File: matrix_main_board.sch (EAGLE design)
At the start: 137 parts, among them IC1 MKE02_44PIN, IC2 24AA01SM, IC3 74HC595D, IC4 74HC595D, IC5 74HC595D, IC6 74HC595D, IC7 NPIC6C596, IC8 NPIC6C596, IC9 W25Q128, U1 RP2040

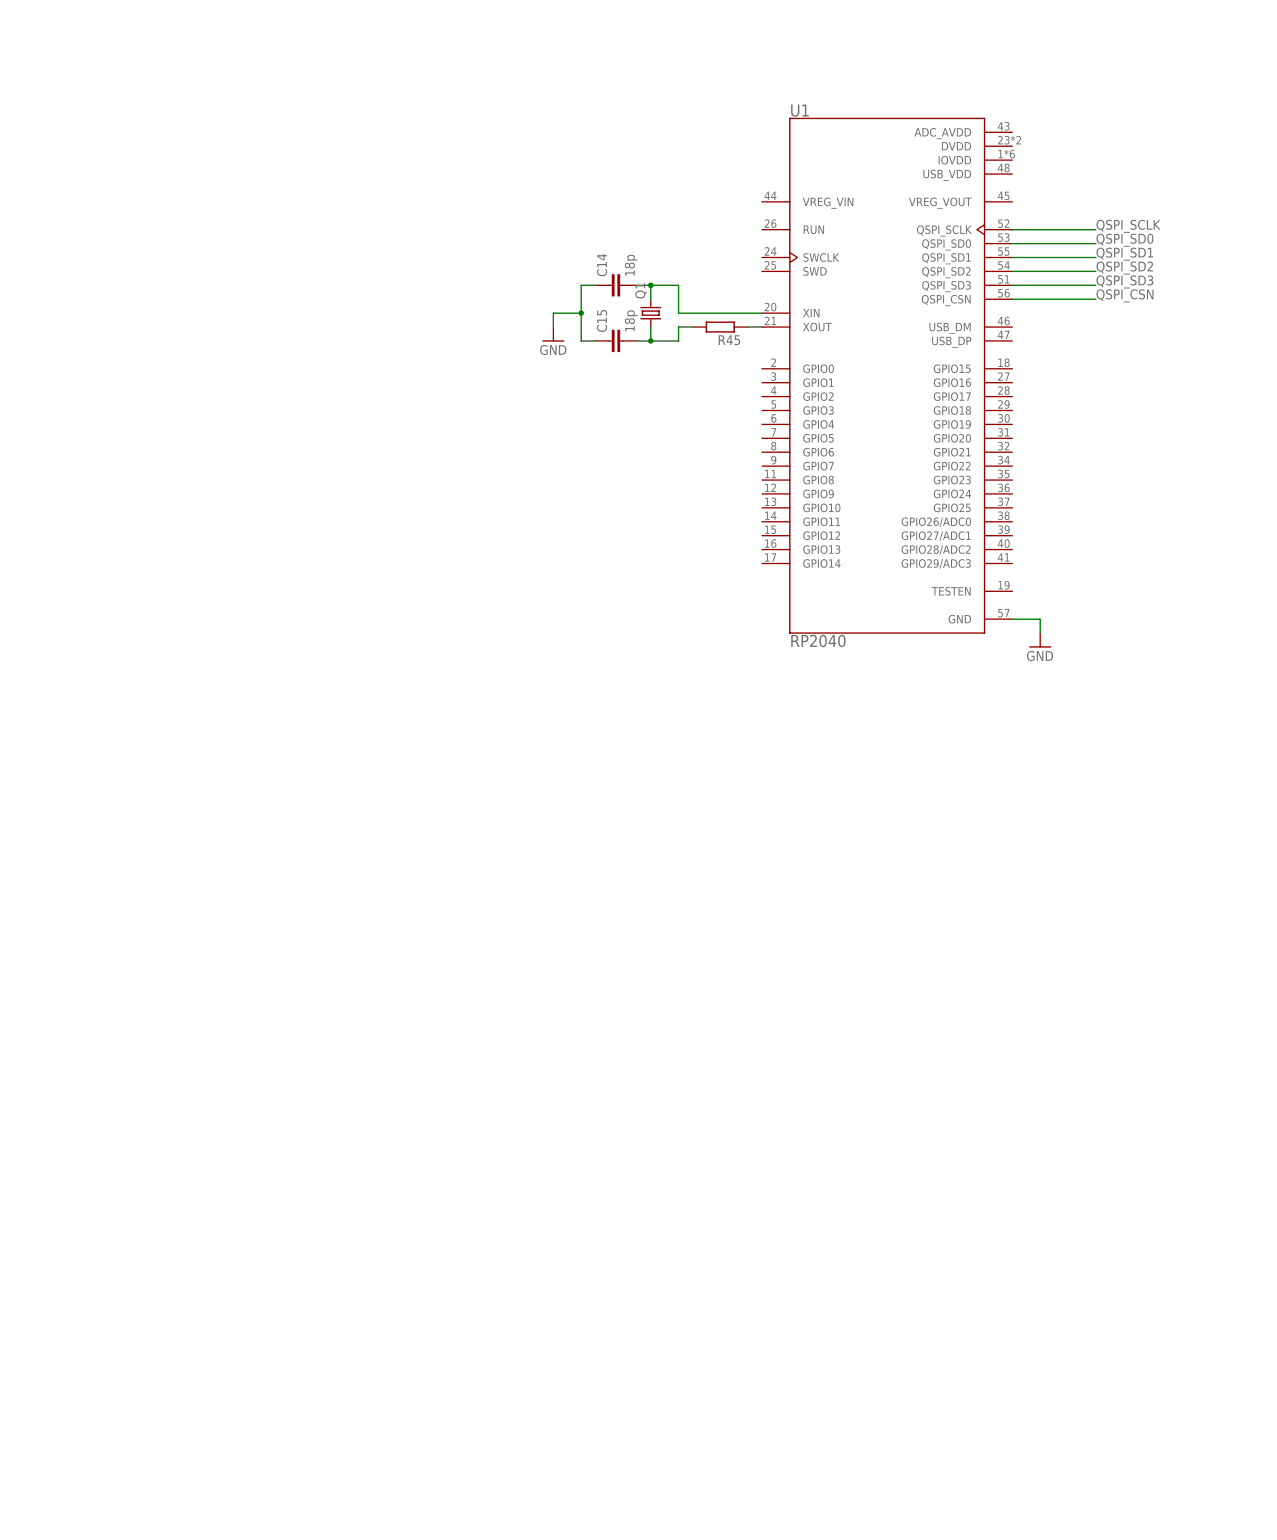
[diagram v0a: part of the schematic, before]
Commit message: ASAS
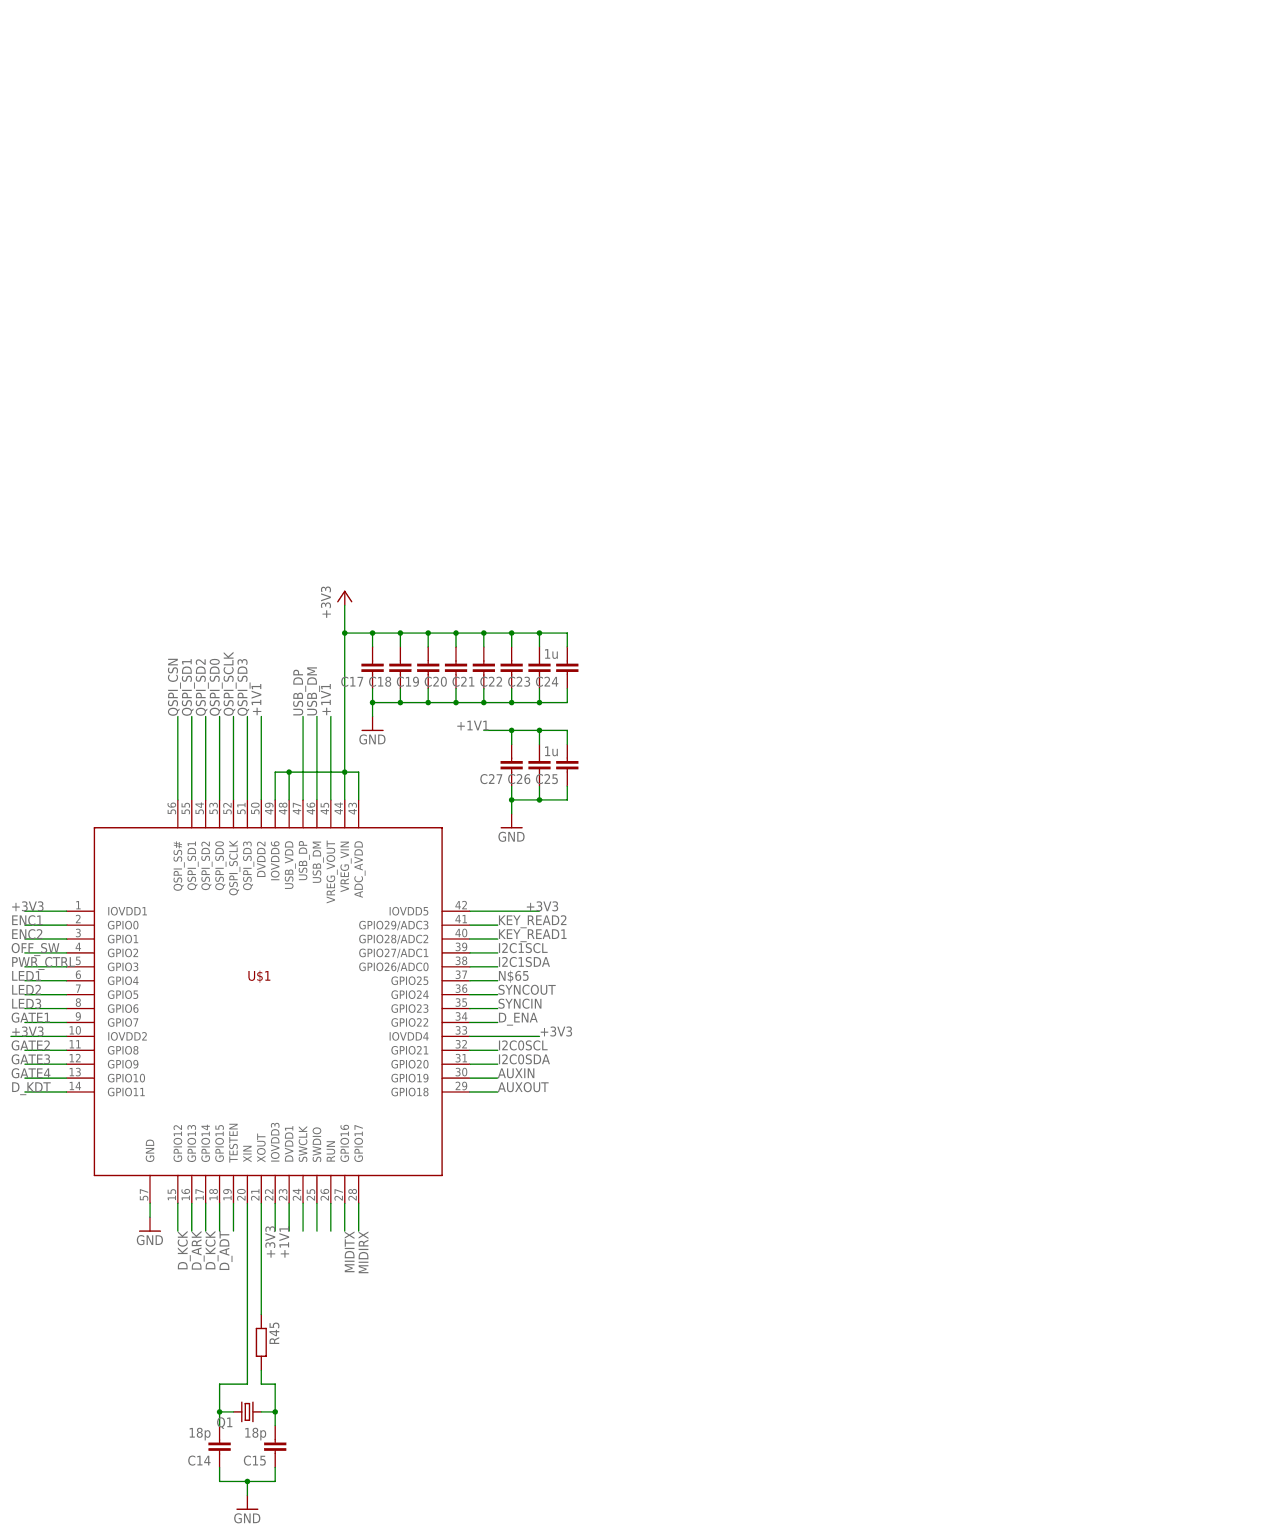
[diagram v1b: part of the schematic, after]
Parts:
- removed U1: RP2040, RP2040:RP2040
- added C17, C18, C19, C20, C21, C22, C23, C26, C27: (no value), rcl:C-EUC0805
- added C24, C25: 1u, rcl:C-EUC0805
- added U$1: RP2040, jason_eagle6:RP2040
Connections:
- new net +1V1: C25.2, C26.2, C27.2, U$1.DVDD1, U$1.DVDD2, U$1.VREG_VOUT
- new net +3V3: C17.2, C18.2, C19.2, C20.2, C21.2, C22.2, C23.2, C24.2, U$1.ADC_AVDD, U$1.IOVDD1, U$1.IOVDD2, U$1.IOVDD3, U$1.IOVDD4, U$1.IOVDD5, U$1.IOVDD6, U$1.USB_VDD, U$1.VREG_VIN
- new net N$44: U$1.TESTEN
- new net N$45: U$1.SWCLK
- new net N$46: U$1.SWDIO
- new net N$47: U$1.RUN
- new net N$65: U$1.GPIO25
- new net USB_DM: U$1.USB_DM
- new net USB_DP: U$1.USB_DP
- net AUXIN: now also U$1.GPIO19
- net AUXOUT: now also U$1.GPIO18
- net D_ADT: now also U$1.GPIO15
- net D_ARK: now also U$1.GPIO13
- net D_ENA: now also U$1.GPIO22
- net D_KCK: now also U$1.GPIO12, U$1.GPIO14
- net D_KDT: now also U$1.GPIO11
- net ENC1: now also U$1.GPIO0
- net ENC2: now also U$1.GPIO1
- net GATE1: now also U$1.GPIO7
- net GATE2: now also U$1.GPIO8
- net GATE3: now also U$1.GPIO9
- net GATE4: now also U$1.GPIO10
- net GND: now also C17.1, C18.1, C19.1, C20.1, C21.1, C22.1, C23.1, C24.1, C25.1, C26.1, C27.1, U$1.GND; no longer U1.GND
- net I2C0SCL: now also U$1.GPIO21
- net I2C0SDA: now also U$1.GPIO20
- net I2C1SCL: now also U$1.GPIO27/ADC1
- net I2C1SDA: now also U$1.GPIO26/ADC0
- net KEY_READ1: now also U$1.GPIO28/ADC2
- net KEY_READ2: now also U$1.GPIO29/ADC3
- net LED1: now also U$1.GPIO4
- net LED2: now also U$1.GPIO5
- net LED3: now also U$1.GPIO6
- net MIDIRX: now also U$1.GPIO17
- net MIDITX: now also U$1.GPIO16
- net N$10: now also U$1.XIN; no longer U1.XIN
- net N$15: now also U$1.XOUT; no longer U1.XOUT
- net OFF_SW: now also U$1.GPIO2
- net PWR_CTRL: now also U$1.GPIO3
- net QSPI_CSN: now also U$1.QSPI_SS#; no longer U1.QSPI_CSN
- net QSPI_SCLK: now also U$1.QSPI_SCLK; no longer U1.QSPI_SCLK
- net QSPI_SD0: now also U$1.QSPI_SD0; no longer U1.QSPI_SD0
- net QSPI_SD1: now also U$1.QSPI_SD1; no longer U1.QSPI_SD1
- net QSPI_SD2: now also U$1.QSPI_SD2; no longer U1.QSPI_SD2
- net QSPI_SD3: now also U$1.QSPI_SD3; no longer U1.QSPI_SD3
- net SYNCIN: now also U$1.GPIO23
- net SYNCOUT: now also U$1.GPIO24
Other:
- moved on the sheet: C14, C15, Q1, R45
